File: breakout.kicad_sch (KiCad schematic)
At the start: 5 parts, among them U1 STS4X

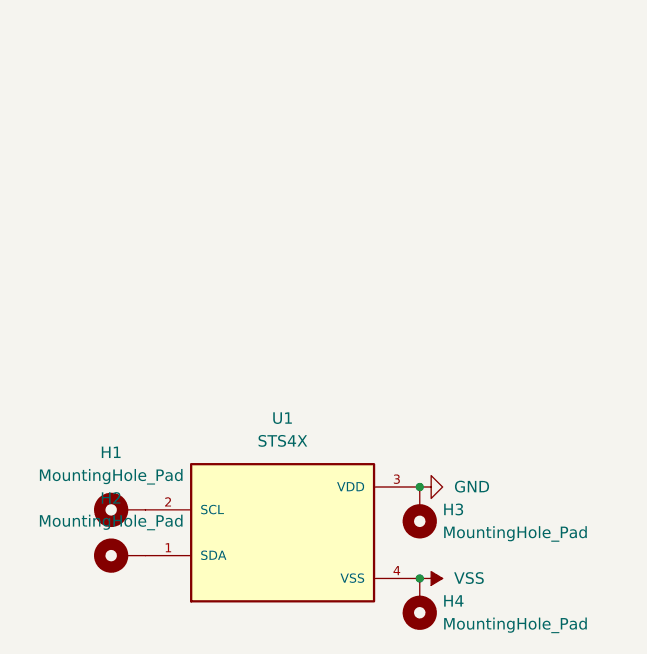
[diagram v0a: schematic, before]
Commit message: put the projects into one
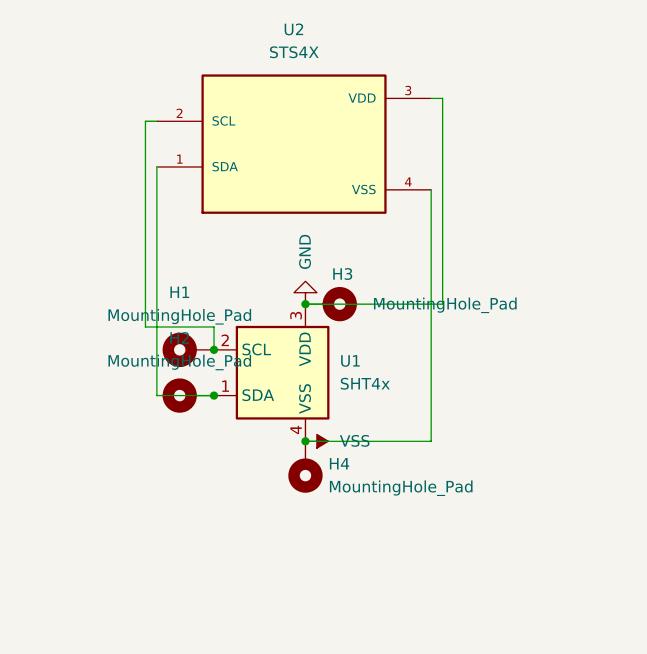
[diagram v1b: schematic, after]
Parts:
- removed U1: STS4X, STS4X:STS4X, symbol STS4X:STS4X
- added U1: SHT4x, Sensor_Humidity:Sensirion_DFN-4_1.5x1.5mm_P0.8mm_SHT4x_NoCentralPad, symbol Sensor_Humidity:SHT4x
- added U2: STS4X, STS4X:STS4X, symbol STS4X:STS4X
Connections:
- net GND: now also U1.3 (VDD), U2.3 (VDD)
- net VSS: now also U1.4 (VSS), U2.4 (VSS)
- net at H1.1: now also U1.2 (SCL), U2.2 (SCL)
- net at H2.1: now also U1.1 (SDA), U2.1 (SDA)
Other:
- moved on the sheet: H1, H2, H3, H4
